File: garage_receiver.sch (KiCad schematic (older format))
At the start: 21 parts, among them J1 Conn_01x04_Female, J2 Screw_Terminal_01x04, Q1 2N7002, SW1 SW_DIP_x08, U1 HT12D, U2 MP1470

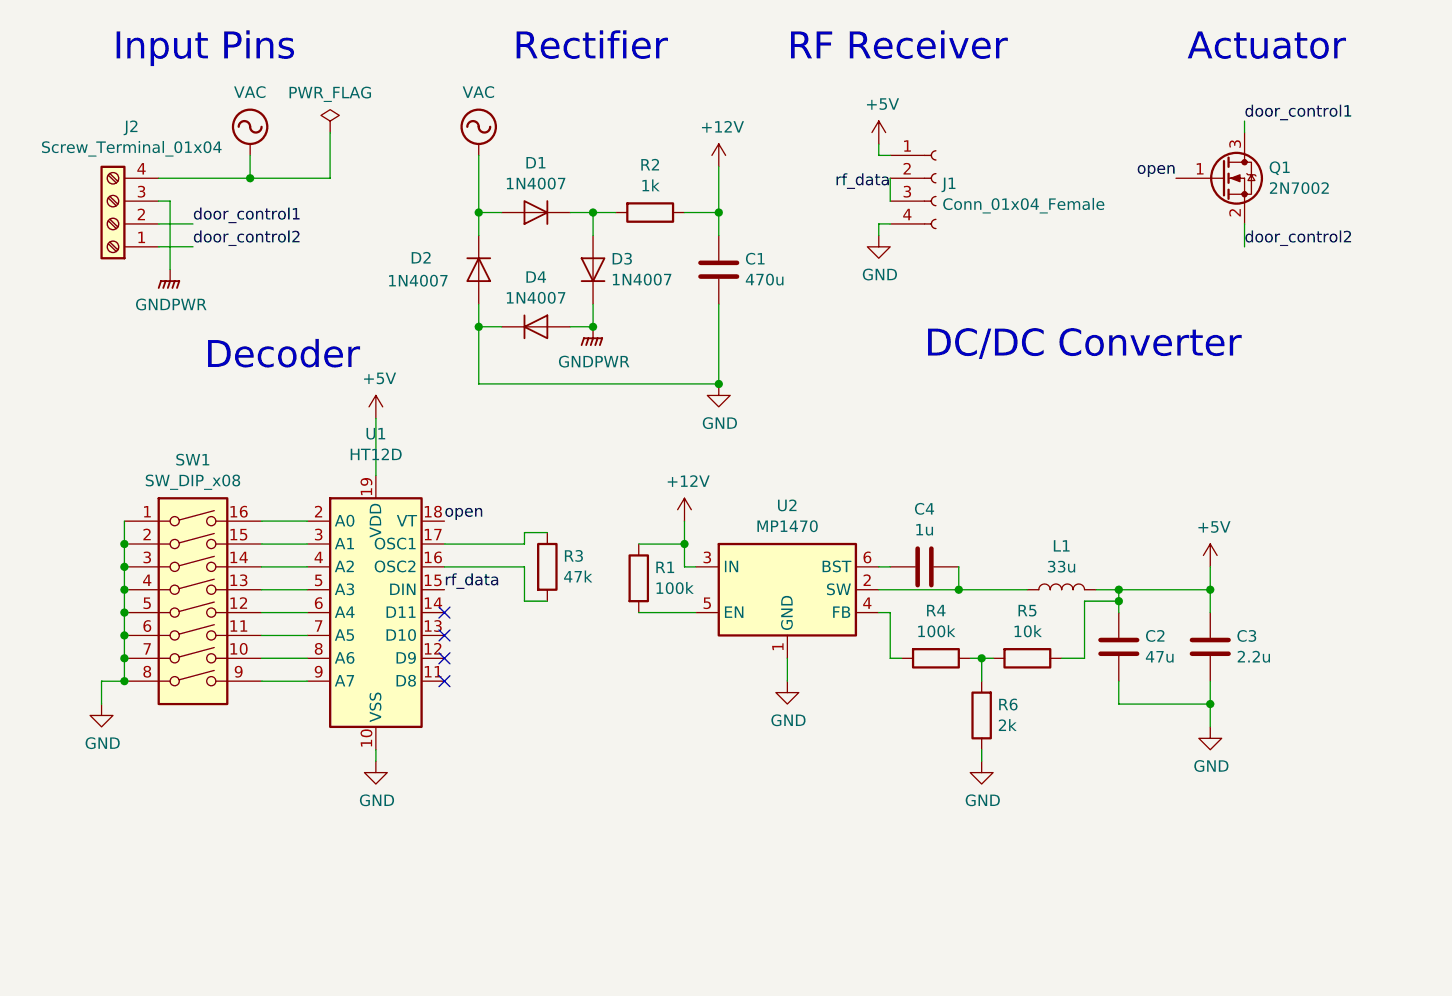
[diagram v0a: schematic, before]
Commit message: Prepare for production
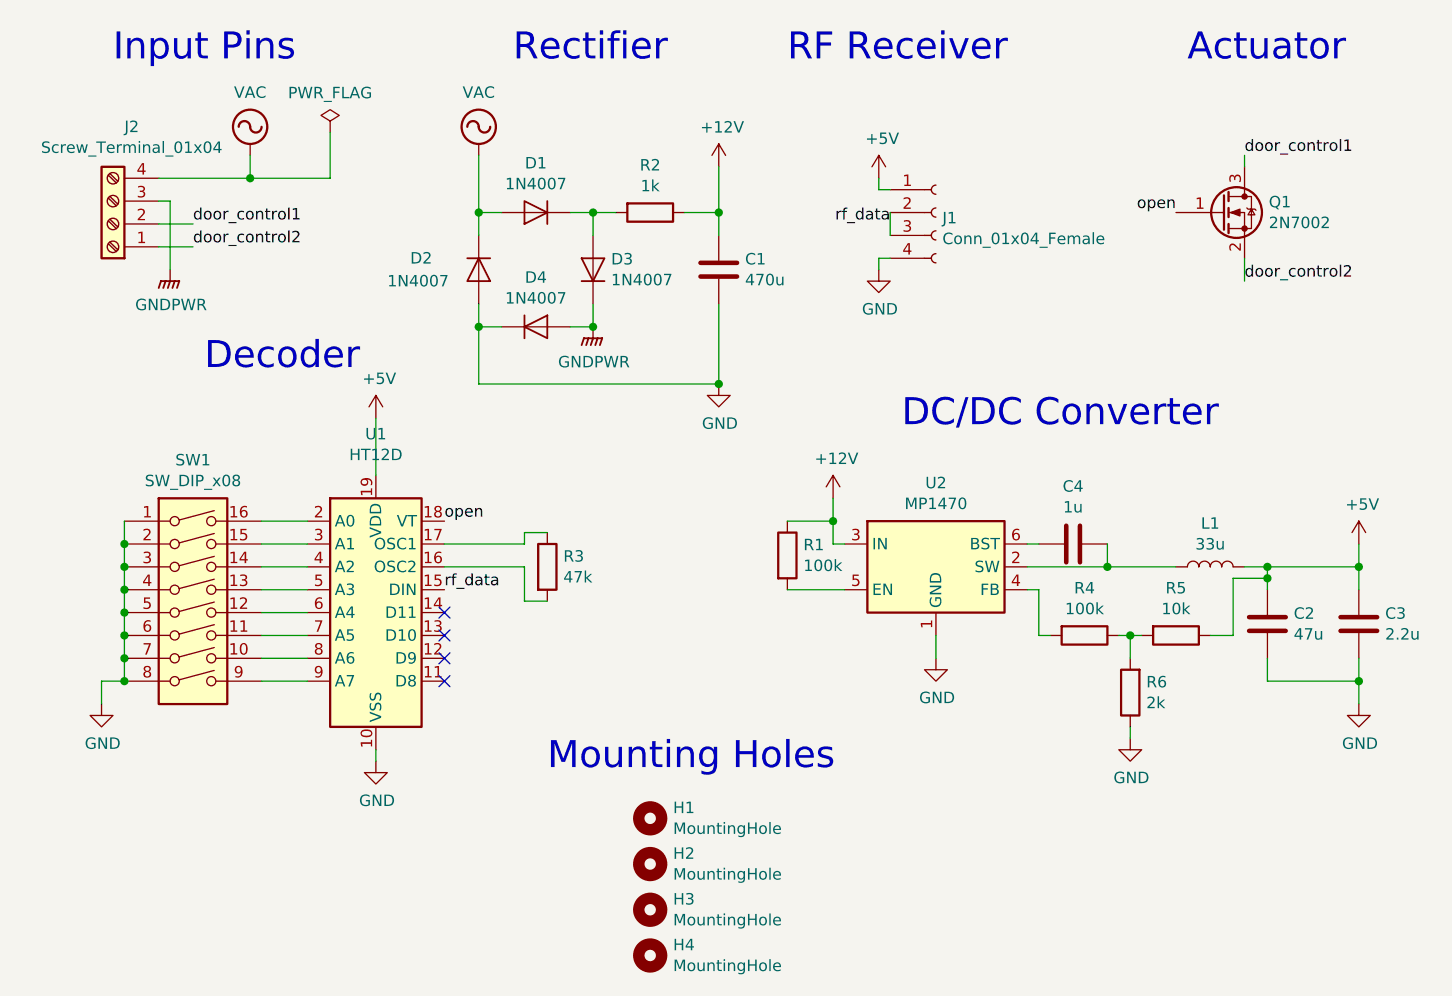
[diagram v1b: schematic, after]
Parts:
- added H1, H2, H3, H4: MountingHole, MountingHole:MountingHole_3.2mm_M3, symbol Mechanical:MountingHole
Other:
- note added: "Mounting Holes"
- moved on the sheet: C2, C3, C4, J1, L1, Q1, R1, R4, R5, R6, U2
